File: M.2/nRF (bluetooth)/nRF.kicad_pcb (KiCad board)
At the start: 2 copper layers, 22 x 26 mm, 21 parts, among them M1 M.2_Key_E, SW101 RESET, U1 MK08, U2 BQ24232HARGTT

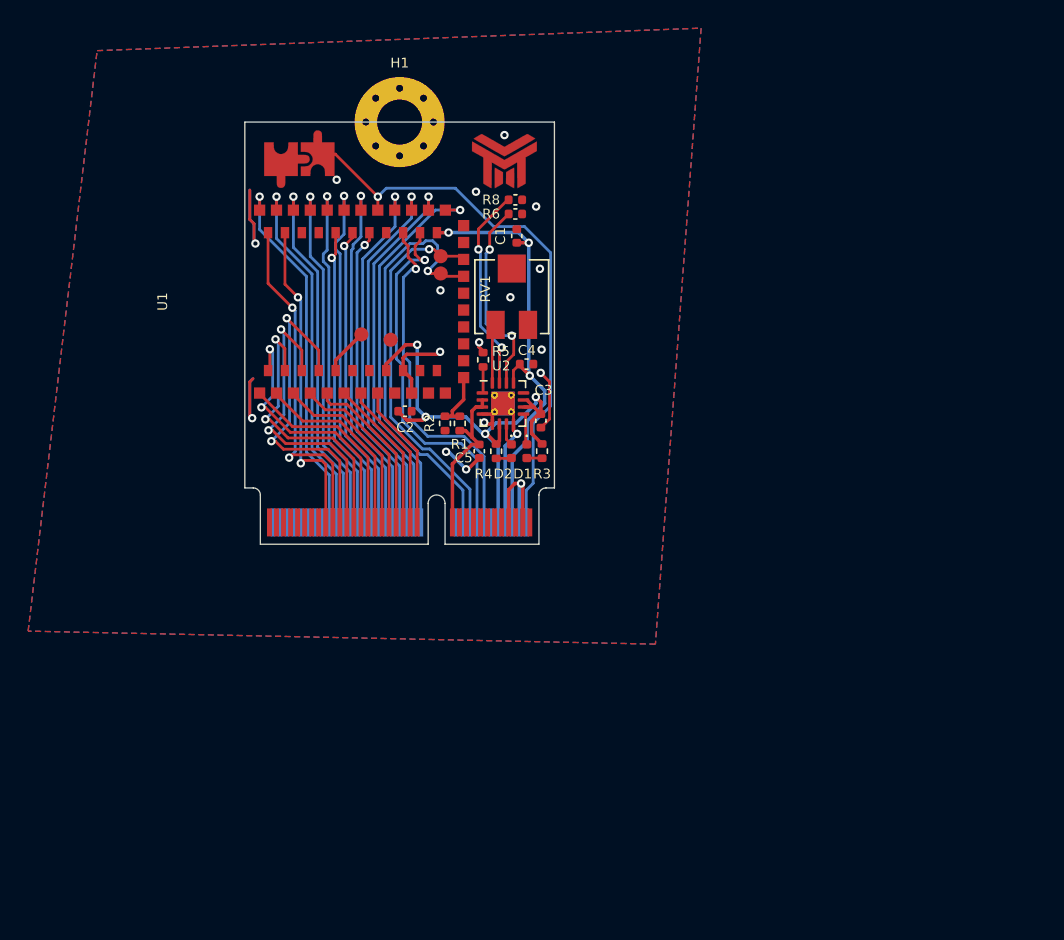
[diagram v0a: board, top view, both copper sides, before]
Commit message: prettify files a lil bit
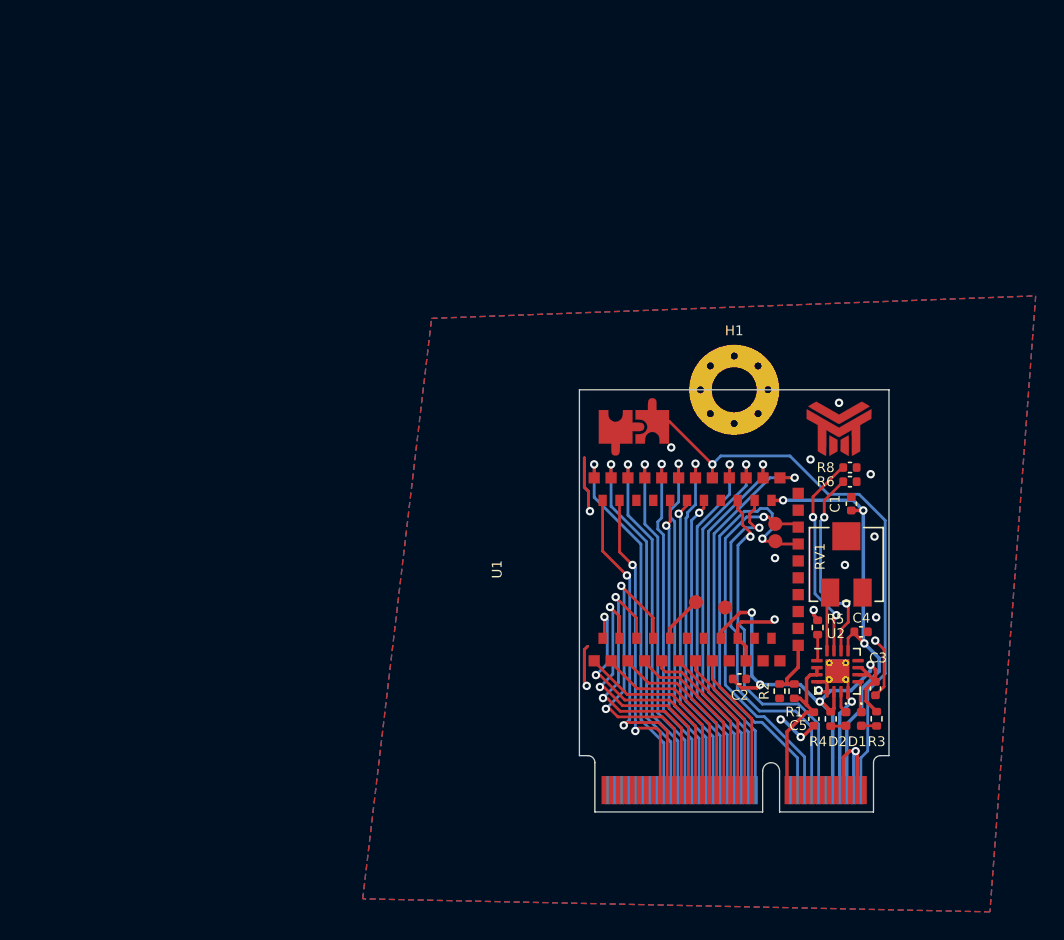
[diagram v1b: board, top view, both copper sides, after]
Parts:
- moved L1 30.4 mm to (42.2, 21.8)
- moved R3 30.4 mm to (44.9, 42.4)
- moved C2 30.4 mm to (35.1, 39.6)
- moved C3 30.4 mm to (44.8, 40.3)
- moved C4 30.4 mm to (43.8, 36.2)
- moved D1 30.4 mm to (43.8, 42.4)
- moved H1 30.4 mm to (34.8, 19.0)
- moved M1 30.4 mm to (34.8, 49.0)
- moved R1 30.4 mm to (39.0, 40.4)
- moved R2 30.4 mm to (38.0, 40.4)
- moved R4 30.4 mm to (41.6, 42.4)
- moved R5 30.4 mm to (40.7, 35.9)
- moved R8 30.4 mm to (43.0, 24.6)
- moved RV1 30.4 mm to (42.7, 31.4)
- moved SW101 30.4 mm to (27.6, 21.6)
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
